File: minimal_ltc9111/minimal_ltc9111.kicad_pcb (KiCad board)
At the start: 4 copper layers, 19.1 x 59.7 mm, 32 parts, among them J1 FW-02-03-G-D-085-155, J2 FW-02-03-G-D-085-155, Q1 100 V, Q2 100 V, Q3 100 V, Q4 100.0 V, U1 LTC9111RDE-PBF

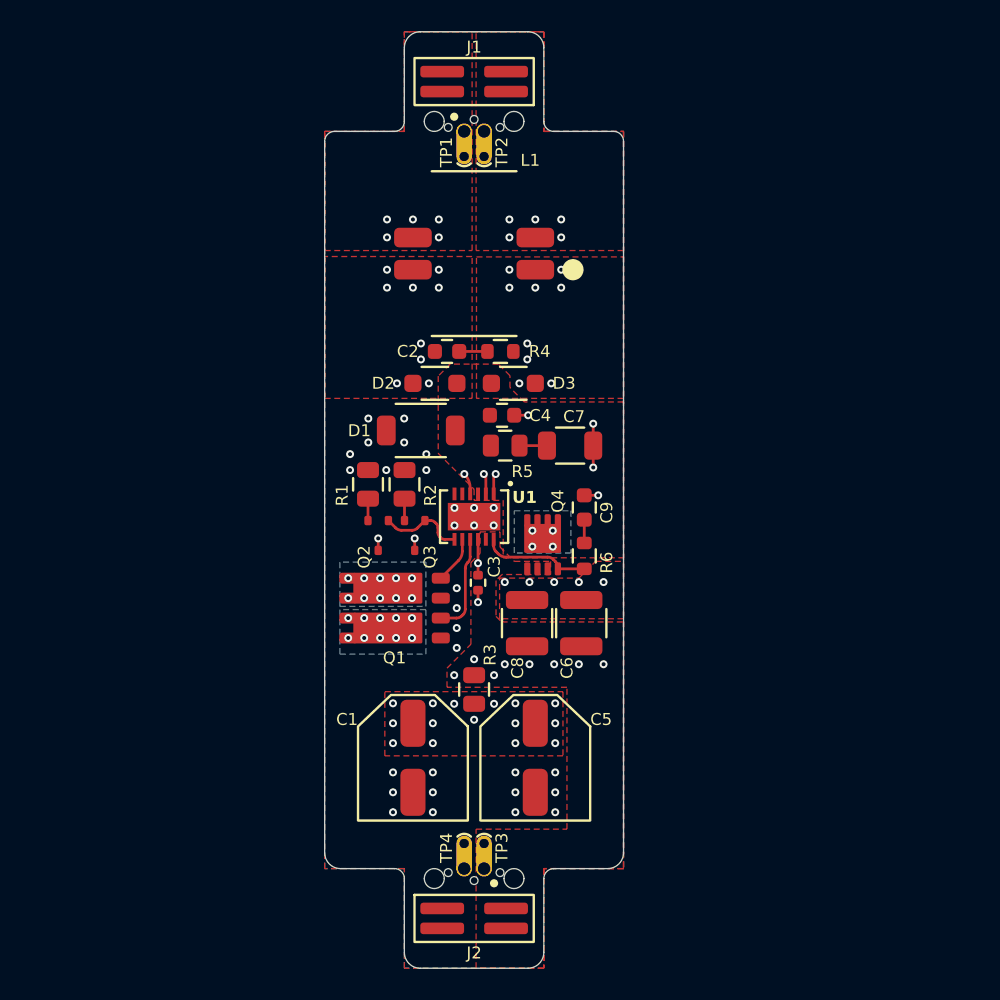
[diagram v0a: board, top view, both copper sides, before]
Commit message: Backup
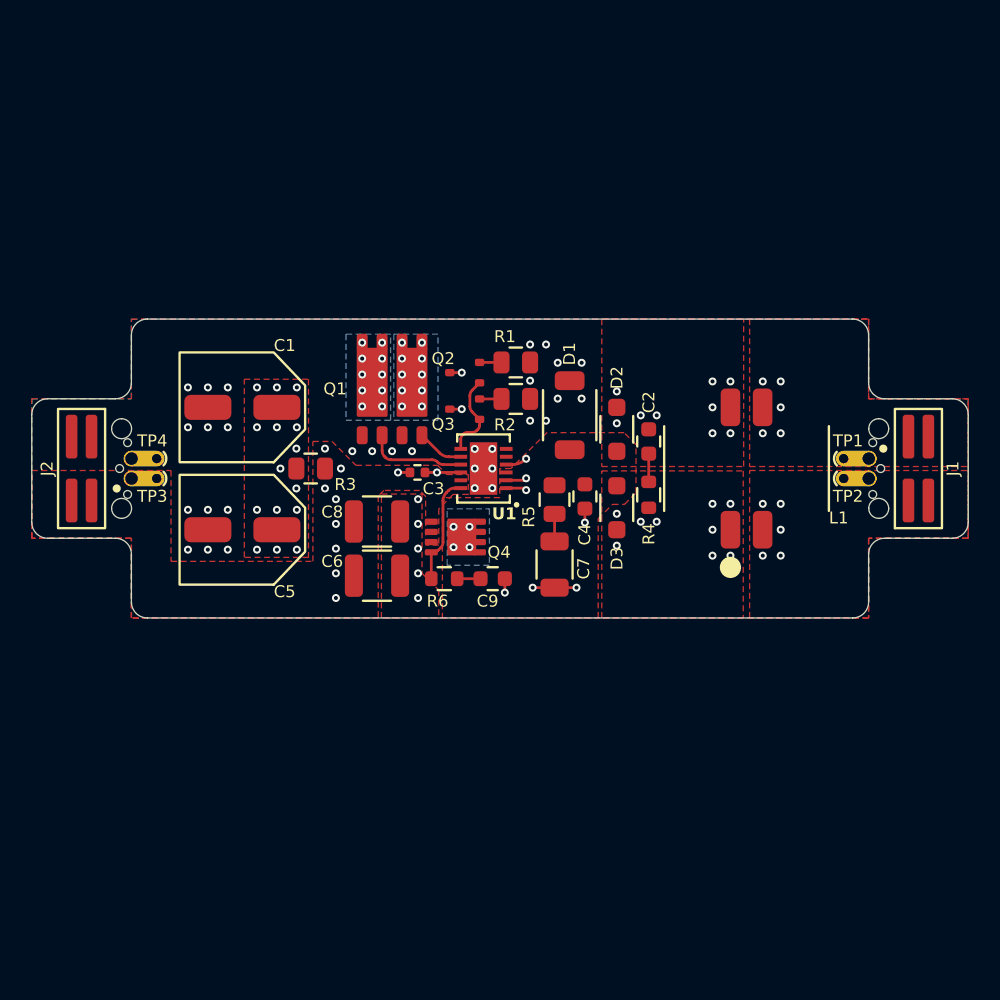
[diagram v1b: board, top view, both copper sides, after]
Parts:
- moved J2 38.1 mm to (128.9, 105.2), turned to 180 degrees
- moved J1 37.6 mm to (182.2, 105.2), turned to 0 degrees
- moved MB2 34.5 mm to (131.5, 105.2), turned to 90 degrees
- moved MB1 34.0 mm to (179.7, 105.2), turned to -90 degrees
- moved TP4 33.7 mm to (132.1, 104.5), turned to 0 degrees
- moved TP3 33.5 mm to (132.1, 105.8), turned to 0 degrees
- moved TP1 33.2 mm to (179.1, 104.5), turned to 180 degrees
- moved TP2 33.0 mm to (179.1, 105.8), turned to 180 degrees
- moved C1 24.8 mm to (139.2, 101.3), turned to 180 degrees
- moved C5 23.7 mm to (139.2, 109.1), turned to 180 degrees
- moved L1 22.1 mm to (171.3, 105.2), turned to 90 degrees
- moved R3 17.5 mm to (143.5, 105.2), turned to 180 degrees
- moved C2 14.1 mm to (165.1, 103.4), turned to 90 degrees
- moved Q1 14.0 mm to (148.7, 100.1), turned to 90 degrees
- moved C6 13.4 mm to (147.7, 112.0), turned to 0 degrees
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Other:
- board size 19.1 x 59.7 mm -> 59.7 x 19 mm

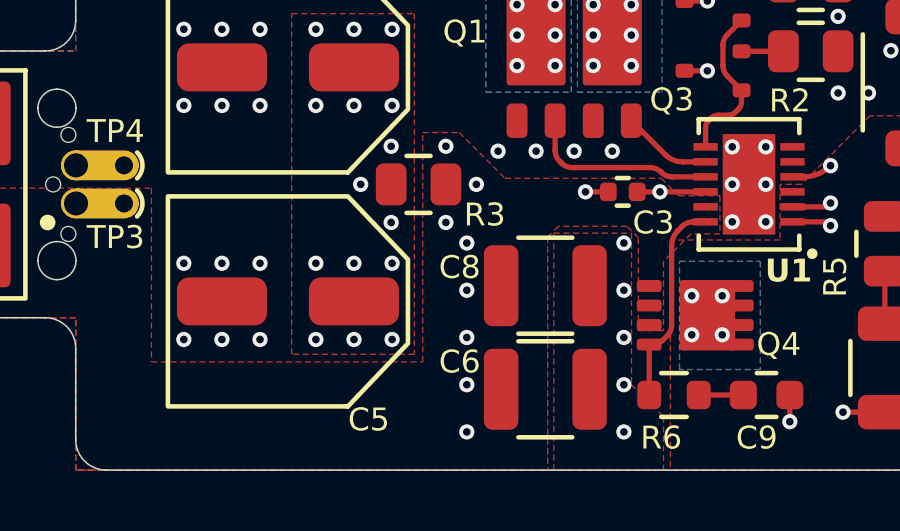
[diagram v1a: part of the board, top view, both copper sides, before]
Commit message: Backup
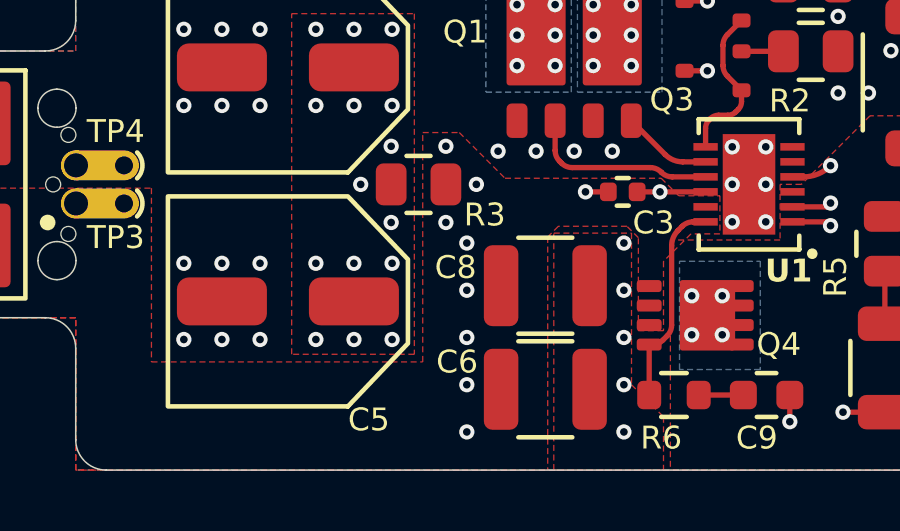
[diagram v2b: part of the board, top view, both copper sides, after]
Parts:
- C6, C8: footprint capacitor_footprints:C_1210_3225Metric -> capacitor_footprints:C_1210_200_3225Metric
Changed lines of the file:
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@@
 		)
 	)
-	(footprint "capacitor_footprints:C_1210_3225Metric"
+	(footprint "capacitor_footprints:C_1210_200_3225Metric"
 		(layer "F.Cu")
 		(at 147.735077 108.533755)
 		(property "Reference" "C8"
-			(at -2.1572 -0.608838 0)
+			(at -2.294677 -0.609155 0)
 			(unlocked yes)
 			(layer "F.SilkS")
@@
 			)
 		)
-		(property "Footprint" "capacitor_footprints:C_1210_3225Metric"
+		(property "Footprint" "capacitor_footprints:C_1210_200_3225Metric"
 			(at 0 0 0)
 			(layer "F.Fab")
@@
 			)
 		)
-		(property "Description" "CAP SMD 4.7 µF X7S 10% 1210 100V"
+		(property "Description" "CAP SMD 4.7 µF X7S 10% 1210_200 100V"
 			(at 0 0 0)
 			(layer "F.Fab")
@@
 			)
 		)
-		(property "Case Code - in" "1210"
+		(property "Case Code - in" "1210_200"
 			(at 0 0 0)
 			(unlocked yes)
@@
 		)
 		(property "Voltage Rating" "100V"
+			(at 0 0 0)
+			(unlocked yes)
+			(layer "F.Fab")
+			(hide yes)
+			(effects
+				(font
+					(size 1 1)
+					(thickness 0.15)
+				)
+			)
+		)
+		(property "3dviewer Link" "https://3dviewer.net/index.html#model=https://github.com/ionutms/KiCAD_Symbols_Generator/blob/main/3D_models/C_1210.step"
+			(at 0 0 0)
+			(unlocked yes)
+			(layer "F.Fab")
+			(hide yes)
+			(effects
+				(font
+					(size 1 1)
+					(thickness 0.15)
+				)
+			)
+		)
+		(property "Capacitor Type" "Ceramic"
 			(at 0 0 0)
 			(unlocked yes)
@@
 			(net 16 "/OUT")
 			(pintype "unspecified")
-			(teardrops
-				(best_length_ratio 0.5)
-				(max_length 1)
-				(best_width_ratio 1)
-				(max_width 2)
-				(curve_points 5)
-				(filter_ratio 0.9)
-				(enabled yes)
-				(allow_two_segments yes)
-				(prefer_zone_connections yes)
-			)
 		)
 		(pad "2" smd roundrect
@@
 			(net 3 "GND")
 			(pintype "unspecified")
-			(teardrops
-				(best_length_ratio 0.5)
-				(max_length 1)
-				(best_width_ratio 1)
-				(max_width 2)
-				(curve_points 5)
-				(filter_ratio 0.9)
-				(enabled yes)
-				(allow_two_segments yes)
-				(prefer_zone_connections yes)
-			)
-		)
-		(model "${KIPRJMOD}/KiCAD_Symbol_Generator/3D_models/C_1210.step"
+		)
+		(model "${KIPRJMOD}/KiCAD_Symbol_Generator/3D_models/C_1210_200.step"
 			(offset
 				(xyz 0 0 0)
@@
 		)
 	)
-	(footprint "capacitor_footprints:C_1210_3225Metric"
+	(footprint "capacitor_footprints:C_1210_200_3225Metric"
 		(layer "F.Cu")
 		(at 147.735077 111.986885)
 		(property "Reference" "C6"
-			(at -2.1572 -0.912368 0)
+			(at -2.243877 -0.912685 0)
 			(unlocked yes)
 			(layer "F.SilkS")
@@
 			)
 		)
-		(property "Footprint" "capacitor_footprints:C_1210_3225Metric"
+		(property "Footprint" "capacitor_footprints:C_1210_200_3225Metric"
 			(at 0 0 0)
 			(layer "F.Fab")
@@
 			)
 		)
-		(property "Description" "CAP SMD 4.7 µF X7S 10% 1210 100V"
+		(property "Description" "CAP SMD 4.7 µF X7S 10% 1210_200 100V"
 			(at 0 0 0)
 			(layer "F.Fab")
@@
 			)
 		)
-		(property "Case Code - in" "1210"
+		(property "Case Code - in" "1210_200"
 			(at 0 0 0)
 			(unlocked yes)
@@
 		)
 		(property "Voltage Rating" "100V"
+			(at 0 0 0)
+			(unlocked yes)
+			(layer "F.Fab")
+			(hide yes)
+			(effects
+				(font
+					(size 1 1)
+					(thickness 0.15)
+				)
+			)
+		)
+		(property "3dviewer Link" "https://3dviewer.net/index.html#model=https://github.com/ionutms/KiCAD_Symbols_Generator/blob/main/3D_models/C_1210.step"
+			(at 0 0 0)
+			(unlocked yes)
+			(layer "F.Fab")
+			(hide yes)
+			(effects
+				(font
+					(size 1 1)
+					(thickness 0.15)
+				)
+			)
+		)
+		(property "Capacitor Type" "Ceramic"
 			(at 0 0 0)
 			(unlocked yes)
@@
 			(net 16 "/OUT")
 			(pintype "unspecified")
-			(teardrops
-				(best_length_ratio 0.5)
-				(max_length 1)
-				(best_width_ratio 1)
-				(max_width 2)
-				(curve_points 5)
-				(filter_ratio 0.9)
-				(enabled yes)
-				(allow_two_segments yes)
-				(prefer_zone_connections yes)
-			)
 		)
 		(pad "2" smd roundrect
@@
 			(net 3 "GND")
 			(pintype "unspecified")
-			(teardrops
-				(best_length_ratio 0.5)
-				(max_length 1)
-				(best_width_ratio 1)
-				(max_width 2)
-				(curve_points 5)
-				(filter_ratio 0.9)
-				(enabled yes)
-				(allow_two_segments yes)
-				(prefer_zone_connections yes)
-			)
-		)
-		(model "${KIPRJMOD}/KiCAD_Symbol_Generator/3D_models/C_1210.step"
+		)
+		(model "${KIPRJMOD}/KiCAD_Symbol_Generator/3D_models/C_1210_200.step"
 			(offset
 				(xyz 0 0 0)
